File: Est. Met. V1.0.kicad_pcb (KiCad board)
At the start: 2 copper layers, 100 x 100 mm, 18 parts, among them J1 UART, J2 Pluv., J3 PWR, J4 S_Temp, Q1 2N7000, U1 StepDownLM2596, U2 SIM800L_B, U3 BluePill_STM32F103

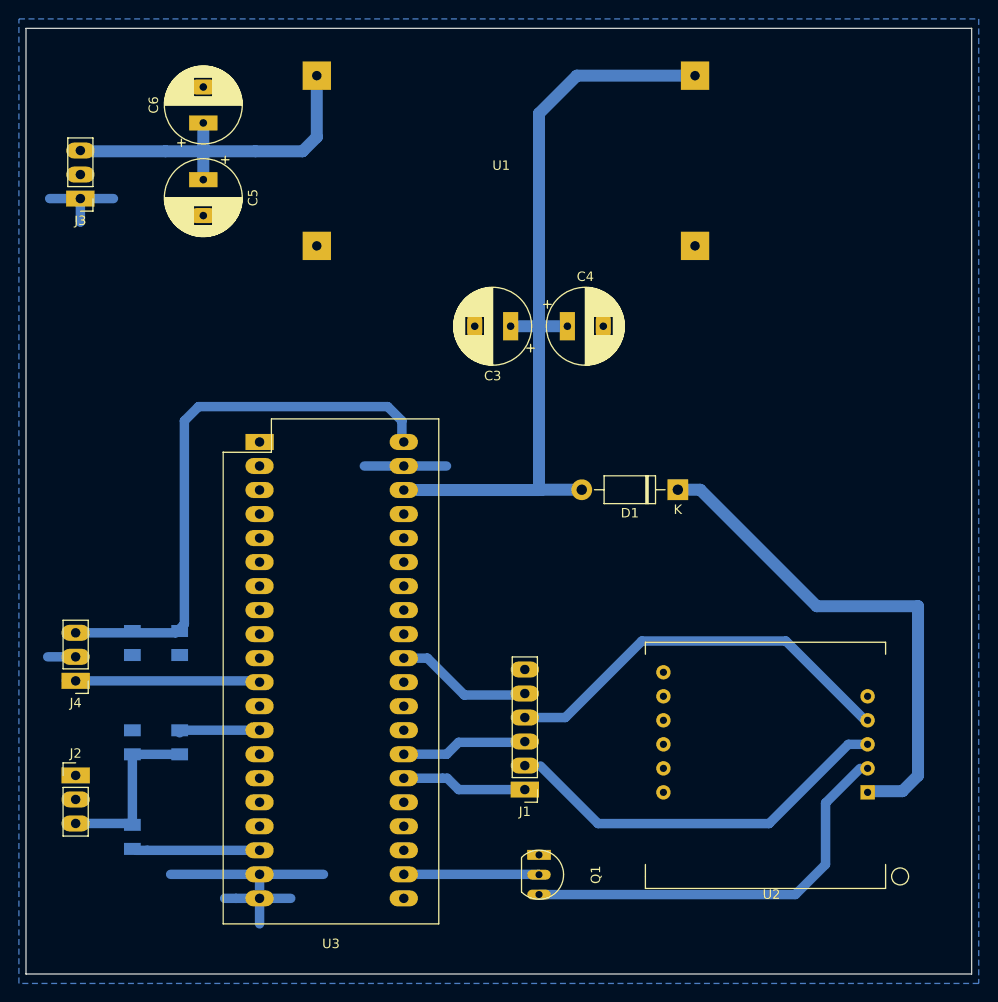
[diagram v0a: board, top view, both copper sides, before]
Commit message: Nueva placa
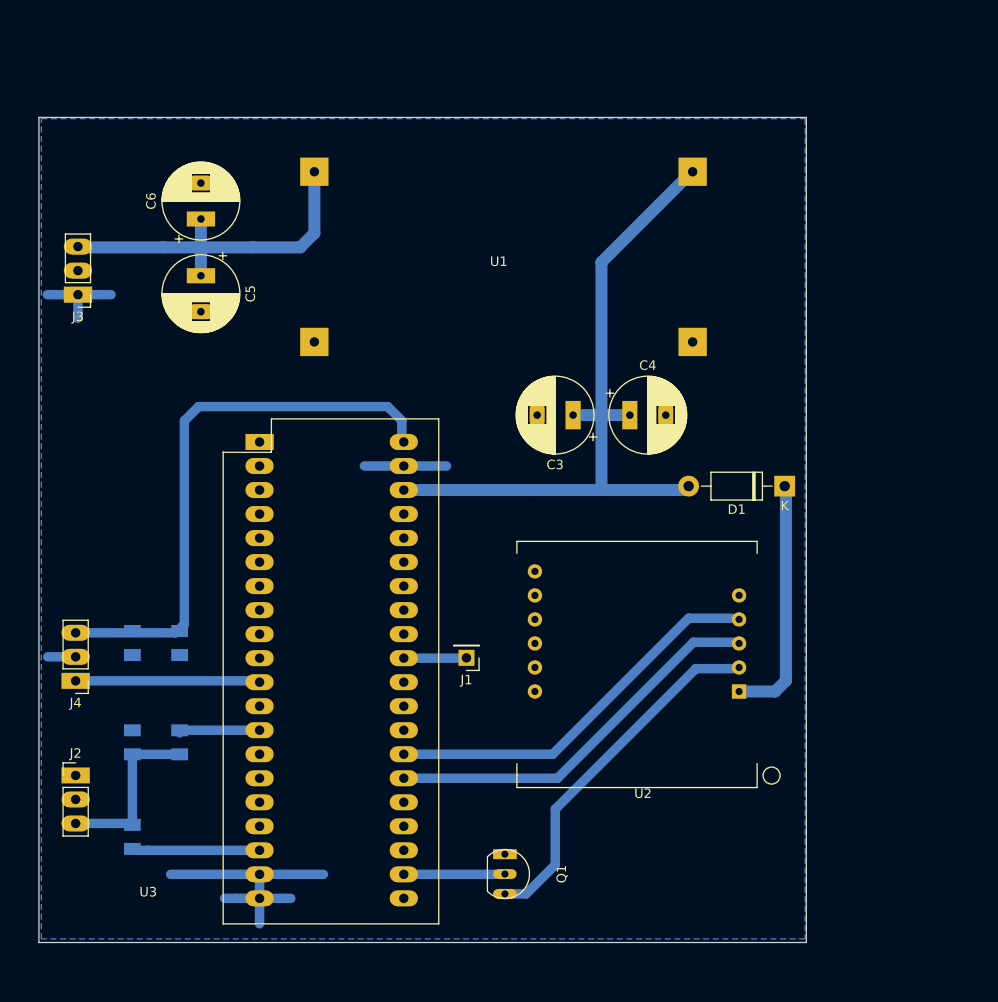
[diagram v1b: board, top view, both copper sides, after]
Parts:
- J1: value UART -> Conn_01x01; footprint Connector_PinHeader_2.54mm:PinHeader_1x06_P2.54mm_Vertical -> Connector_PinHeader_2.54mm:PinHeader_1x01_P2.54mm_Vertical
- moved U2 17.3 mm to (111.0, 118.7)
- moved J1 15.2 mm to (92.3, 107.6)
- moved C3 11.5 mm to (103.6, 81.9)
- moved C4 11.5 mm to (109.6, 81.9)
- moved D1 11.3 mm to (126.0, 89.4)
- moved C5 10.2 mm to (64.2, 67.2)
- moved C6 10.2 mm to (64.2, 61.2)
- moved J3 10.2 mm to (51.2, 69.2)
- moved U1 10.2 mm to (95.7, 65.2)
- moved Q1 3.61 mm to (96.4, 130.4)
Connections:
- J1 pad 1: TX_MC -> SWO
- U2 pad 4: TX_S800 -> RX_MC
- U3 pad 30: TX_MC -> RX_S800
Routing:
- net TX_S800: track 42.6 -> 0.00 mm
- net +4V: track 53.8 -> 25.9 mm
- net RX_MC: track 12.8 -> 40.7 mm
- net TX_MC: track 12.3 -> 0.00 mm
- net +5V: track 84.1 -> 74.3 mm
- net SWO: track 14.4 -> 6.47 mm
- net RST_S800: track 43.3 -> 37.4 mm
- net MC_RST_S800: track 14.3 -> 9.65 mm
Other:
- board size 100 x 100 mm -> 81.2 x 87.2 mm
